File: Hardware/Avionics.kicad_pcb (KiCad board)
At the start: 4 copper layers, 76 x 76 mm, 0 parts

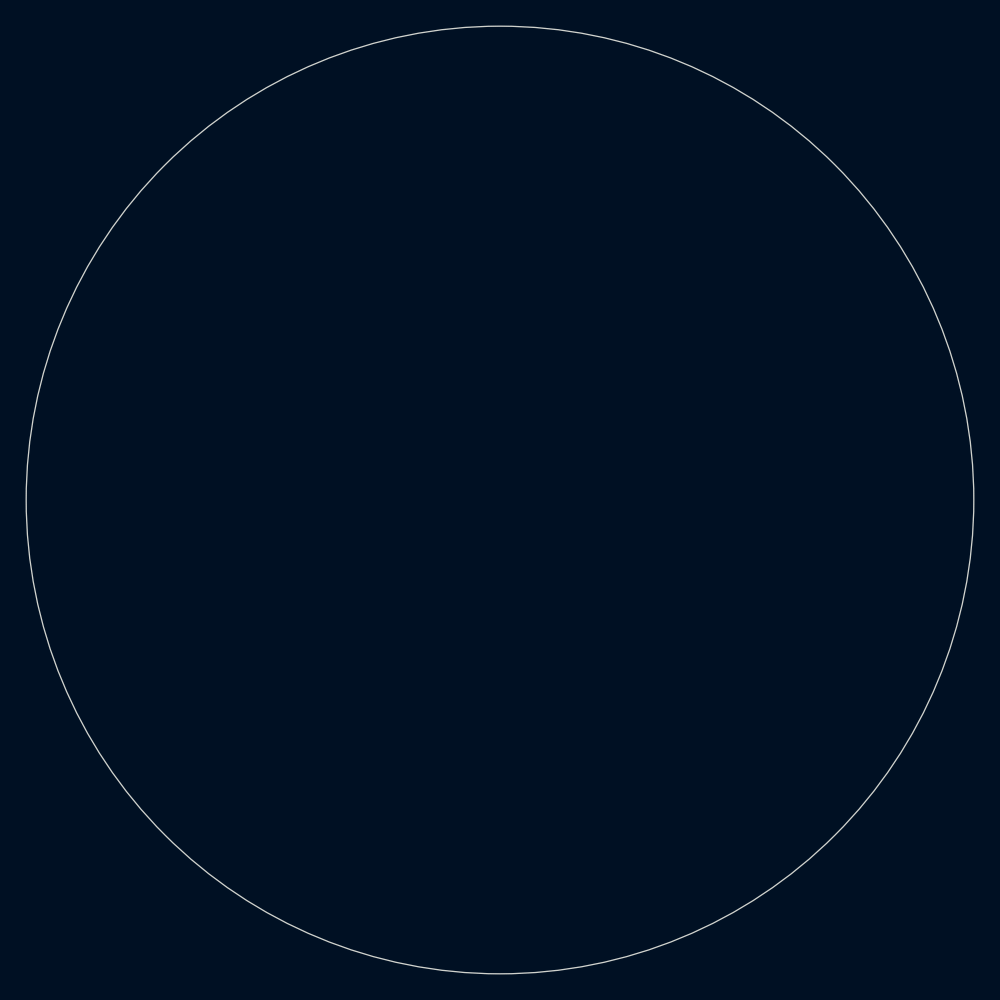
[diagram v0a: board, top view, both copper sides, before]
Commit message: Layout complete, pending review
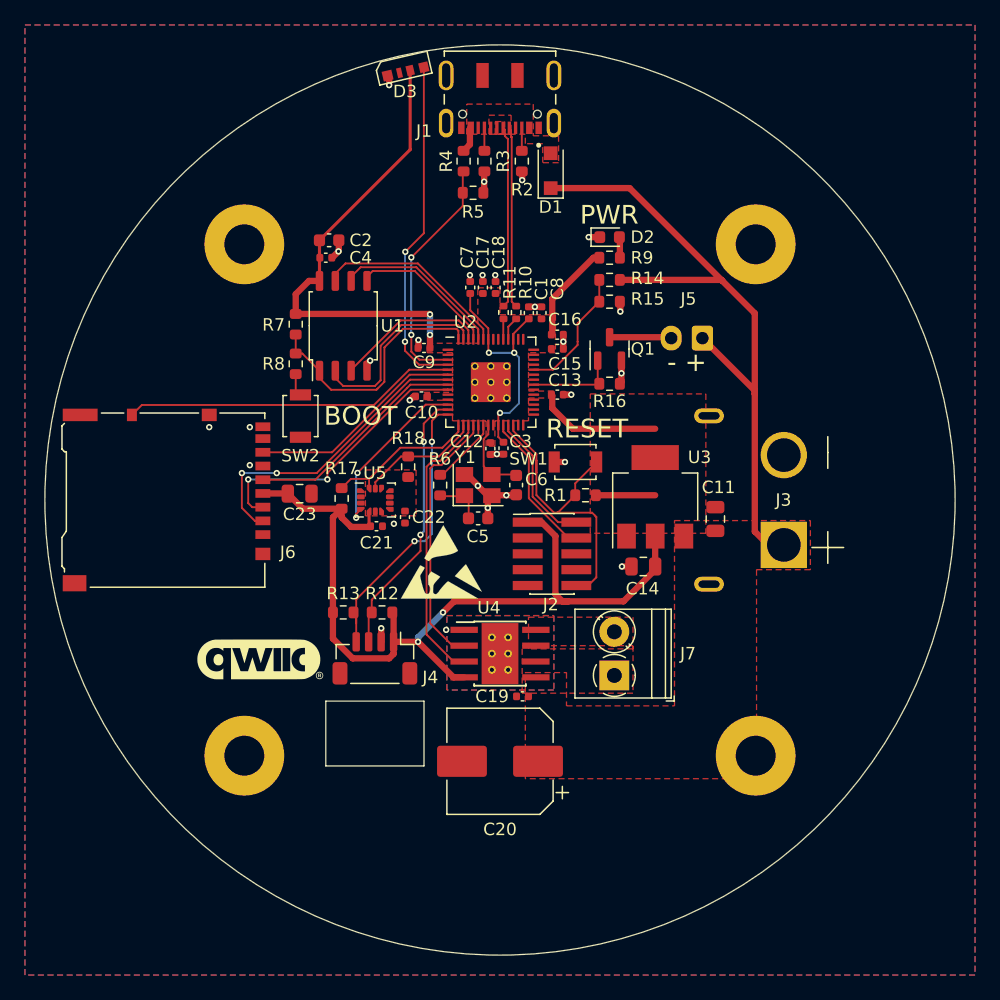
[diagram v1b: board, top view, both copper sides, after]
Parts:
- added C1: 1uF, Capacitor_SMD:C_0402_1005Metric, F.Cu at (154.7, 86.6)
- added C10: 100nF, Capacitor_SMD:C_0402_1005Metric, F.Cu at (146.1, 93.3)
- added C11: 10uF, Capacitor_SMD:C_0805_2012Metric, F.Cu at (169.7, 103.1)
- added C12: 100nF, Capacitor_SMD:C_0402_1005Metric, F.Cu at (151.6, 97.5)
- added C13: 100nF, Capacitor_SMD:C_0402_1005Metric, F.Cu at (157.0, 93.1)
- added C14: 10uF, Capacitor_SMD:C_0805_2012Metric, F.Cu at (163.9, 106.9)
- added C15: 100nF, Capacitor_SMD:C_0402_1005Metric, F.Cu at (157.0, 89.5)
- added C16: 100nF, Capacitor_SMD:C_0402_1005Metric, F.Cu at (157.0, 88.3)
- added C17: 100nF, Capacitor_SMD:C_0402_1005Metric, F.Cu at (151.0, 84.6)
- added C18: 100nF, Capacitor_SMD:C_0402_1005Metric, F.Cu at (152.0, 84.6)
- added C19: 100nF, Capacitor_SMD:C_0402_1005Metric, F.Cu at (154.2, 117.3)
- added C2: 2.2uF, Capacitor_SMD:C_0603_1608Metric, F.Cu at (138.7, 80.8)
- added C20: 100uF, Capacitor_SMD:CP_Elec_8x6.5, F.Cu at (152.4, 122.6)
- added C21: 100nF, Capacitor_SMD:C_0402_1005Metric, F.Cu at (142.5, 103.7)
- added C22: 100nF, Capacitor_SMD:C_0402_1005Metric, F.Cu at (144.8, 103.0)
- added C23: 10uF, Capacitor_SMD:C_0805_2012Metric, F.Cu at (136.3, 101.1)
- added C3: 100nF, Capacitor_SMD:C_0402_1005Metric, F.Cu at (152.7, 97.4)
- added C4: 100nF, Capacitor_SMD:C_0402_1005Metric, F.Cu at (138.4, 82.2)
- added C5: 27pF, Capacitor_SMD:C_0603_1608Metric, F.Cu at (150.6, 103.1)
- added C6: 27pF, Capacitor_SMD:C_0603_1608Metric, F.Cu at (153.7, 100.4)
- added C7: 100nF, Capacitor_SMD:C_0402_1005Metric, F.Cu at (150.0, 84.6)
- added C8: 1uF, Capacitor_SMD:C_0402_1005Metric, F.Cu at (155.7, 86.6)
- added C9: 100nF, Capacitor_SMD:C_0402_1005Metric, F.Cu at (146.3, 89.4)
- added D1: MBR120, Diode_SMD:D_SOD-123F, F.Cu at (156.5, 75.2)
- added D2: PWR, LED_SMD:LED_0603_1608Metric, F.Cu at (161.2, 80.5)
- added D3: SK6812BSIDE, SK6812B:SK6812B_Side, F.Cu at (144.7, 67.3)
- added G***: LOGO, Silkscreen:Qwiic, F.Cu at (133.1, 114.3)
- added G***: LOGO, Silkscreen:WSGC, B.Cu at (147.4, 101.6)
- added G***: LOGO, Silkscreen:MSOE, B.Cu at (132.4, 101.6)
- added H1: M3, MountingHole:MountingHole_3.2mm_M3_Pad, F.Cu at (131.9, 81.1)
- added H2: M3, MountingHole:MountingHole_3.2mm_M3_Pad, F.Cu at (172.9, 81.1)
- added H3: M3, MountingHole:MountingHole_3.2mm_M3_Pad, F.Cu at (172.9, 122.1)
- added H4: M3, MountingHole:MountingHole_3.2mm_M3_Pad, F.Cu at (131.9, 122.1)
- added J1: DX07S016JA1R1500, DX07S016JA1R1500:DX07S016JA1R1500, F.Cu at (152.4, 70.7)
- added J2: SWD, Connector_PinHeader_1.27mm:PinHeader_2x05_P1.27mm_Vertical_SMD, F.Cu at (156.6, 105.9)
- added J3: LiPo 4s, XT60PW-M:AMASS_XT60PW-M, B.Cu at (169.2, 101.6)
- added J4: Qwiic, Connector_JST:JST_SH_BM04B-SRSS-TB_1x04-1MP_P1.00mm_Vertical, F.Cu at (142.4, 114.3)
- added J5: PS-562Q, Connector_JST:JST_XH_B2B-XH-A_1x02_P2.50mm_Vertical, B.Cu at (168.6, 88.6)
- added J6: DM3AT-SF-PEJM5, Connector_Card:microSD_HC_Hirose_DM3AT-SF-PEJM5, F.Cu at (125.7, 101.6)
- added J7: XD-3420, TerminalBlock_Phoenix:TerminalBlock_Phoenix_PT-1,5-2-3.5-H_1x02_P3.50mm_Horizontal, F.Cu at (161.5, 113.9)
- added Q1: BSS138, Package_TO_SOT_SMD:SOT-23, F.Cu at (161.2, 89.5)
- added R1: 10KΩ, Resistor_SMD:R_0603_1608Metric, F.Cu at (159.3, 101.2)
- added R10: 27Ω, Resistor_SMD:R_0402_1005Metric, F.Cu at (153.7, 86.6)
- added R11: 27Ω, Resistor_SMD:R_0402_1005Metric, F.Cu at (152.7, 86.6)
- added R12: 2.2KΩ, Resistor_SMD:R_0603_1608Metric, F.Cu at (142.9, 110.6)
- added R13: 2.2KΩ, Resistor_SMD:R_0603_1608Metric, F.Cu at (139.8, 110.6)
- added R14: 47KΩ, Resistor_SMD:R_0603_1608Metric, F.Cu at (161.2, 83.9)
- added R15: 10KΩ, Resistor_SMD:R_0603_1608Metric, F.Cu at (161.2, 85.7)
- added R16: 10KΩ, Resistor_SMD:R_0603_1608Metric, F.Cu at (161.2, 92.3)
- added R17: 10KΩ, Resistor_SMD:R_0603_1608Metric, F.Cu at (139.7, 101.5)
- added R18: 10KΩ, Resistor_SMD:R_0603_1608Metric, F.Cu at (145.0, 98.9)
- added R2: 5.1KΩ, Resistor_SMD:R_0603_1608Metric, F.Cu at (154.2, 74.4)
- added R3: 5.1KΩ, Resistor_SMD:R_0603_1608Metric, F.Cu at (151.2, 74.4)
- added R4: 5.6KΩ, Resistor_SMD:R_0603_1608Metric, F.Cu at (149.5, 74.4)
- added R5: 10KΩ, Resistor_SMD:R_0603_1608Metric, F.Cu at (150.2, 77.0)
- added R6: 1KΩ, Resistor_SMD:R_0603_1608Metric, F.Cu at (147.6, 100.4)
- added R7: 10KΩ, Resistor_SMD:R_0603_1608Metric, F.Cu at (136.0, 87.5)
- added R8: 1KΩ, Resistor_SMD:R_0603_1608Metric, F.Cu at (136.0, 90.7)
- added R9: 150Ω, Resistor_SMD:R_0603_1608Metric, F.Cu at (161.2, 82.2)
- added REF**: ESD-Logo_6.6x6mm_SilkScreen, Symbol:ESD-Logo_6.6x6mm_SilkScreen, F.Cu at (147.7, 106.6)
- added SW1: RESET, Button_Switch_SMD:SW_SPST_B3U-1000P, F.Cu at (158.4, 98.6)
- added SW2: BOOT, Button_Switch_SMD:SW_SPST_B3U-1000P, F.Cu at (136.4, 94.9)
- added U1: W25Q128JVS, Package_SO:SOIC-8_5.23x5.23mm_P1.27mm, F.Cu at (139.8, 87.6)
- added U2: RP2040, RP2040:RP2040-QFN-56, F.Cu at (151.7, 92.1)
- added U3: NCP1117-3.3, Package_TO_SOT_SMD:SOT-223-3_TabPin2, F.Cu at (164.8, 101.3)
- added U4: DRV8870DDA, Package_SO:Texas_HTSOP-8-1EP_3.9x4.9mm_P1.27mm_EP2.95x4.9mm_Mask2.4x3.1mm_ThermalVias, F.Cu at (152.4, 113.9)
- added U5: LSM6DSO32, Package_LGA:LGA-14_3x2.5mm_P0.5mm_LayoutBorder3x4y, F.Cu at (142.4, 101.6)
- added Y1: 12MHz, Crystal:Crystal_SMD_Abracon_ABM8G-4Pin_3.2x2.5mm, F.Cu at (150.6, 100.4)
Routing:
- net +3V3: track 0.00 -> 131.2 mm, vias 0 -> 4
- net VCC: track 0.00 -> 55.3 mm
- net /RGB_DIN: track 0.00 -> 27.3 mm, vias 0 -> 2
- net /SD_DET: track 0.00 -> 26.8 mm
- net /~{RESET}: track 0.00 -> 25.1 mm
- net GND: track 0.00 -> 24.8 mm, vias 0 -> 28
- net /SDIO_DAT3: track 0.00 -> 24.5 mm, vias 0 -> 2
- net /I2C1_SCL: track 0.00 -> 23.2 mm, vias 0 -> 2
- net /SDIO_CMD: track 0.00 -> 22.5 mm, vias 0 -> 2
- net /MOTOR_PWM1: track 0.00 -> 22.5 mm
- net /I2C1_SDA: track 0.00 -> 21.7 mm, vias 0 -> 2
- net /MOTOR_PWM2: track 0.00 -> 21.2 mm
- net Net-(R7-Pad2): track 0.00 -> 20.5 mm
- net /USB_DET: track 0.00 -> 19.4 mm, vias 0 -> 2
- net +1V1: track 0.00 -> 19.3 mm, vias 0 -> 3
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- added copper zone on F.Cu, net +3V3
- added copper zone on F.Cu, net /USB+
- added copper zone on F.Cu, net /USB-
- added copper zone on B.Cu, net GND
- added copper zone on F.Cu, net GND
- added copper zone on F.Cu, net Net-(J7-Pad1)
- added copper zone on F.Cu, net Net-(J7-Pad2)
- added copper zone on F.Cu, net VBUS
- added copper zone on F.Cu, net VCC
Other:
- board size 76 x 76 mm -> 73 x 73 mm
- rule pad_to_mask_clearance: 0 -> 0.0508
- board text added: "- +"
